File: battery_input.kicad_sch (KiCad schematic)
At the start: 8 parts, among them J4 S2B-PH-SM4, U9 BQ27427

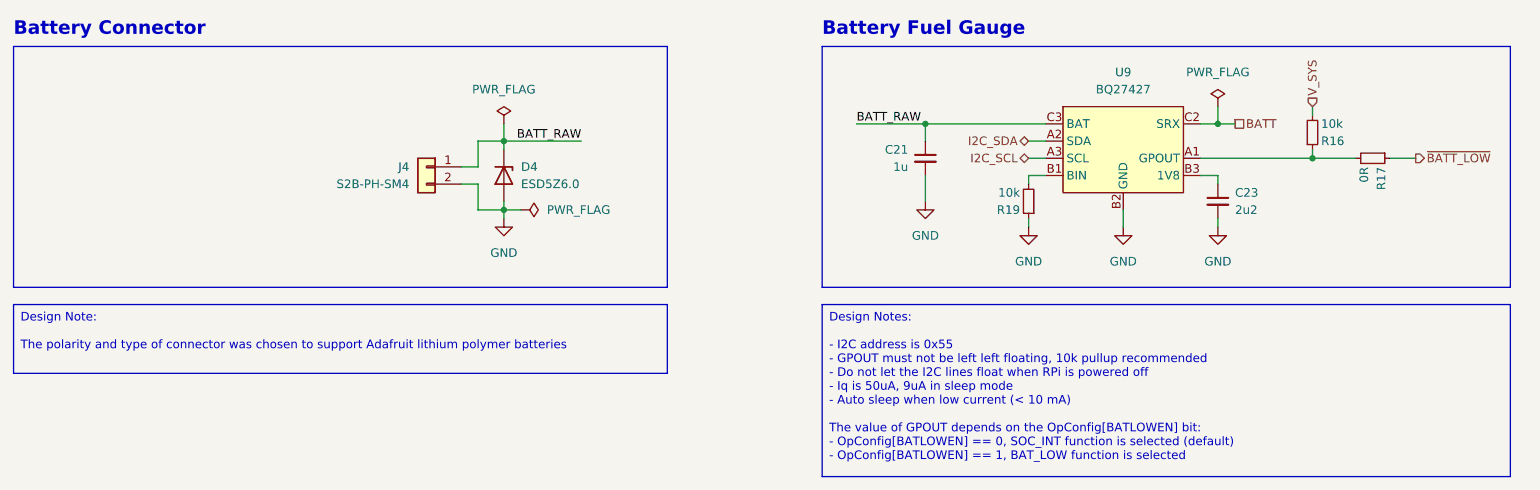
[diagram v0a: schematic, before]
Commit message: finish all schematic changes
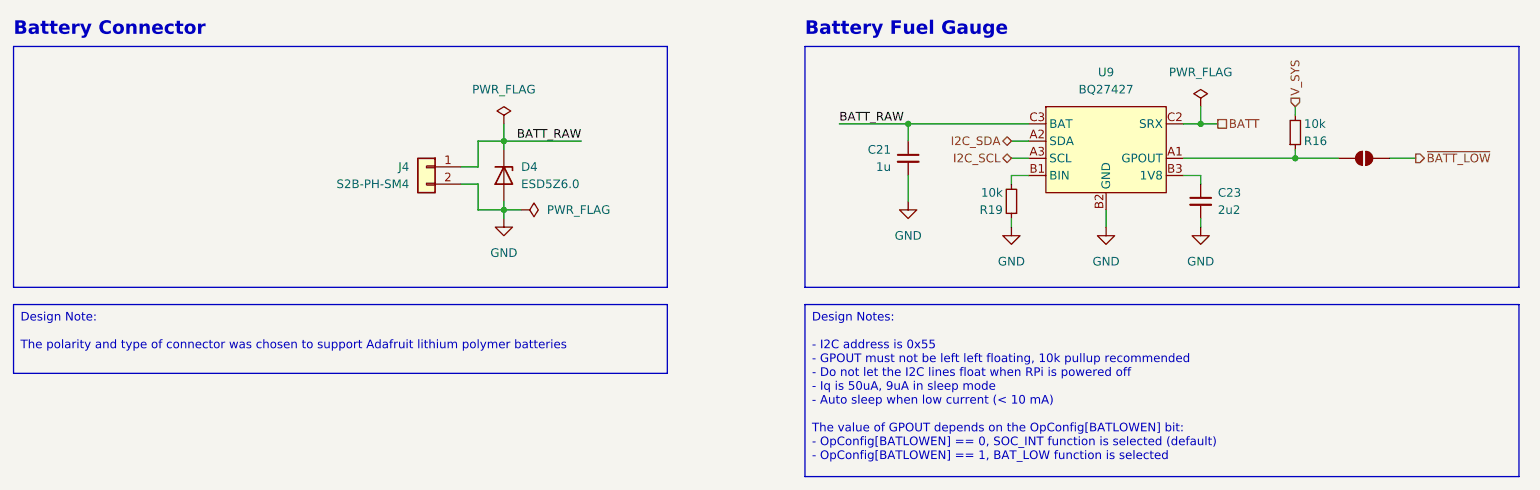
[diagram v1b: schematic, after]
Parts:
- removed R17: 0R, Resistor_SMD:R_0402_1005Metric, symbol Device:R_Small
- added JP1: SolderJumper_2_Open, Jumper:SolderJumper-2_P1.3mm_Open_TrianglePad1.0x1.5mm, symbol Jumper:SolderJumper_2_Open
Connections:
- net ~{BATT_LOW}: now also JP1.2 (B)
- net at R16.1, U9.A1 (GPOUT): now also JP1.1 (A)
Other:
- moved on the sheet: C21, C23, R16, R19, U9
